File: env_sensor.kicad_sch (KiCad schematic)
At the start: 41 parts, among them J1 E Paper, J10 PWMOUT, J15 MH-Z19, J16 ADCs, J18 Conn_01x02_Pin, J3 Barrel_Jack, J4 LED_OUTPUT, J6 ADCs, J7 USB_C_Receptacle_USB2.0_16P, J8 v5_v3, J9 DEBUG, Q1 NMOS, Q2 NMOS, Q3 NMOS, SW1 EN, SW2 BOOT, U3 ESP32-S3-WROOM-1, U4 TXB0104PW, U6 TPS2065CDBV, U7 AP7361C-33E, Y1 Crystal

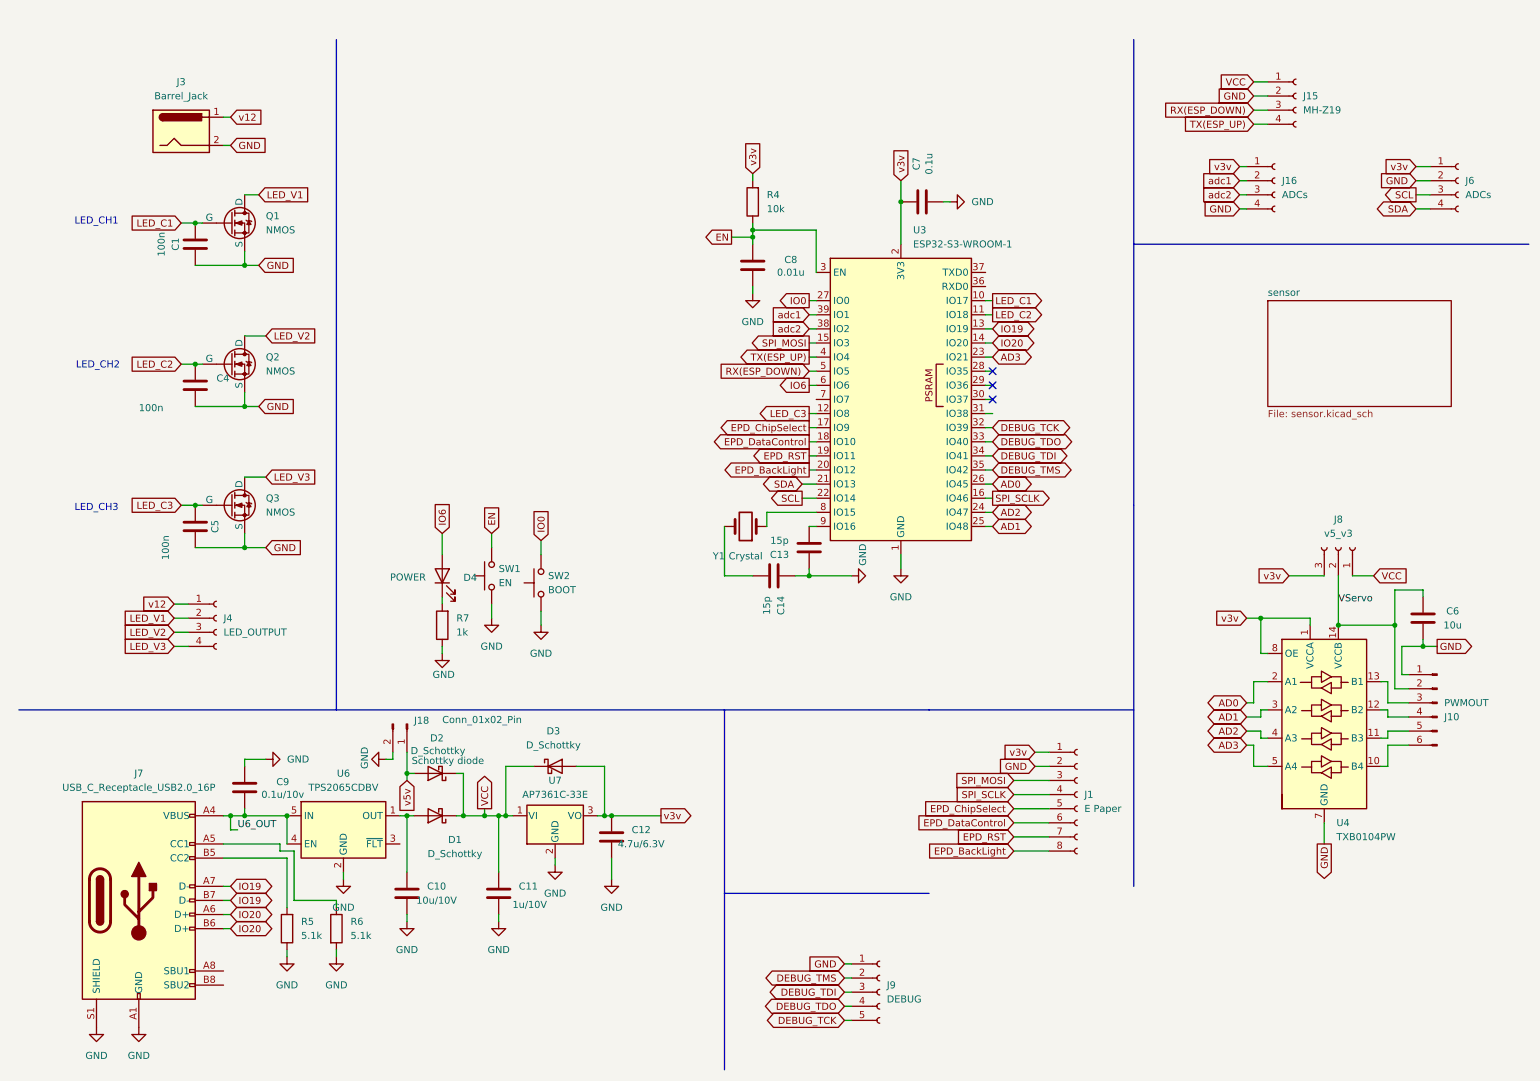
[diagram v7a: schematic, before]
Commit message: update
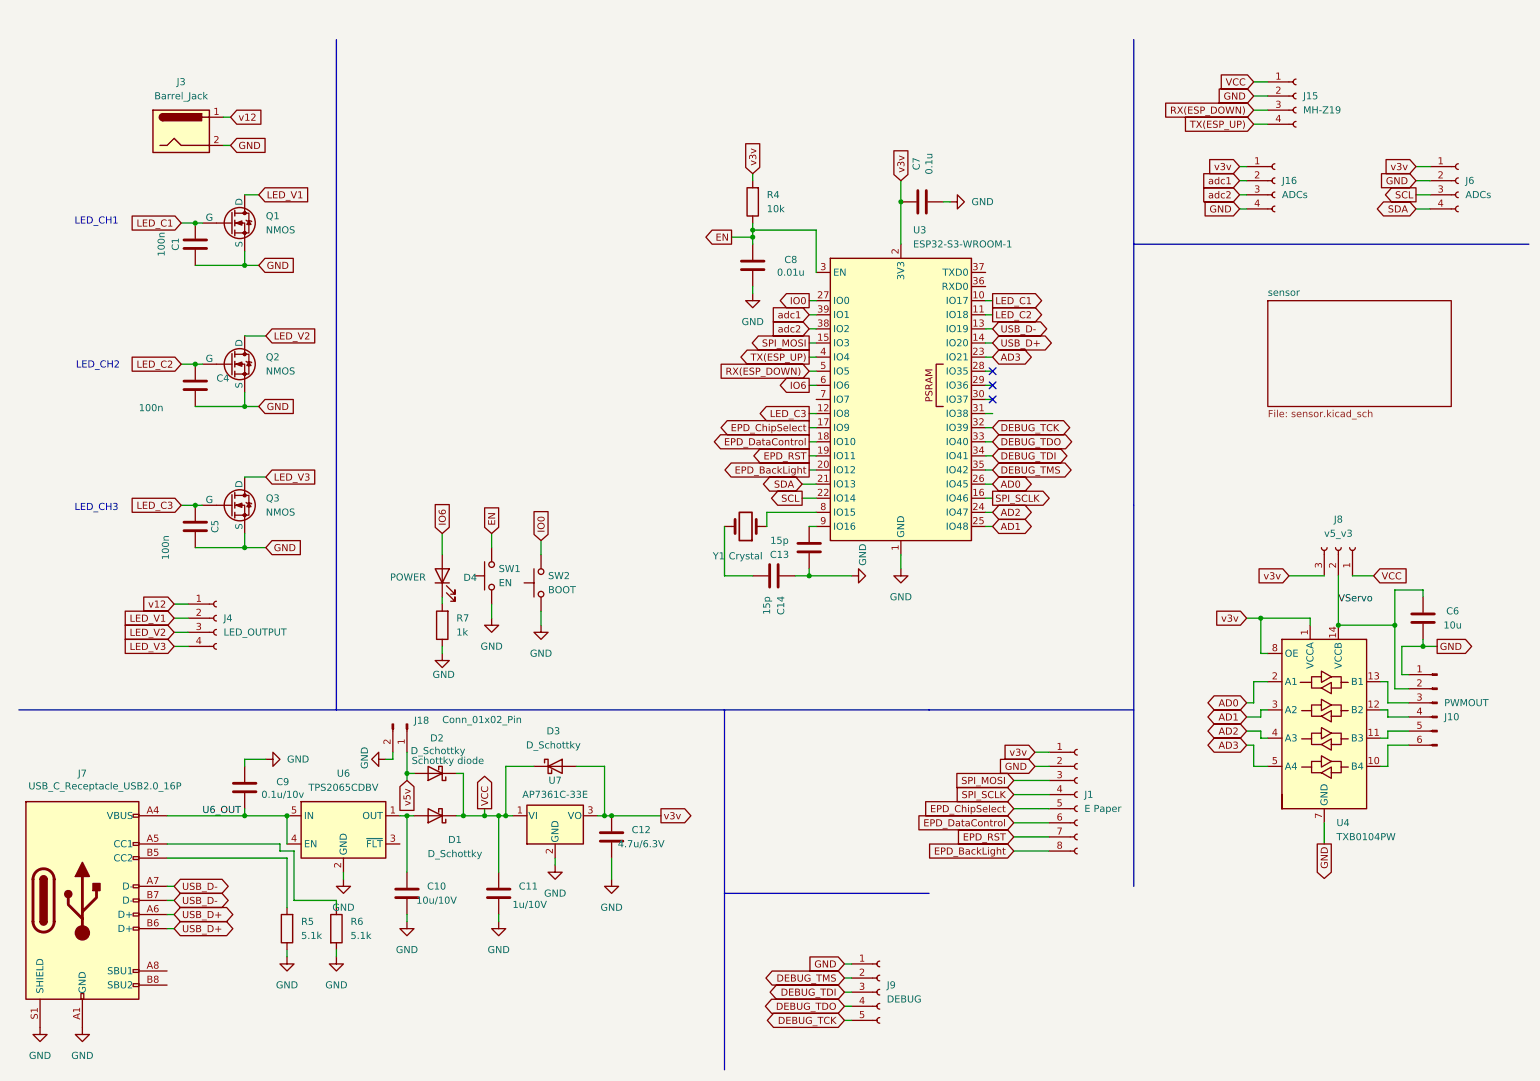
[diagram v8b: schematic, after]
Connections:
- net IO19 renamed USB_D-
- net IO20 renamed USB_D+
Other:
- moved on the sheet: J7
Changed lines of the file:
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@@
 	)
 	(junction
-		(at 50.8 152.4)
-		(diameter 0)
-		(color 0 0 0 0)
-	)
-	(junction
 		(at 171.45 41.91)
 		(diameter 0)
@@
 	(wire
 		(pts
-			(xy 50.8 165.1) (xy 49.53 165.1)
+			(xy 40.64 165.1) (xy 39.37 165.1)
 		)
 		(stroke
@@
 	(wire
 		(pts
-			(xy 53.34 152.4) (xy 50.8 152.4)
-		)
-		(stroke
-			(width 0)
-			(type default)
-		)
-	)
-	(wire
-		(pts
 			(xy 259.08 134.62) (xy 262.89 134.62)
 		)
@@
 	(wire
 		(pts
-			(xy 49.53 160.02) (xy 60.96 160.02)
+			(xy 39.37 160.02) (xy 60.96 160.02)
 		)
 		(stroke
@@
 	(wire
 		(pts
-			(xy 50.8 167.64) (xy 49.53 167.64)
+			(xy 40.64 167.64) (xy 39.37 167.64)
 		)
 		(stroke
@@
 	(wire
 		(pts
+			(xy 39.37 170.18) (xy 40.64 170.18)
+		)
+		(stroke
+			(width 0)
+			(type default)
+		)
+	)
+	(wire
+		(pts
 			(xy 236.22 123.19) (xy 236.22 116.84)
 		)
@@
 	(wire
 		(pts
-			(xy 50.8 172.72) (xy 49.53 172.72)
+			(xy 40.64 172.72) (xy 39.37 172.72)
 		)
 		(stroke
@@
 	(wire
 		(pts
-			(xy 50.8 154.94) (xy 50.8 152.4)
-		)
-		(stroke
-			(width 0)
-			(type default)
-		)
-	)
-	(wire
-		(pts
 			(xy 234.95 27.94) (xy 237.49 27.94)
 		)
@@
 	(wire
 		(pts
-			(xy 50.8 152.4) (xy 49.53 152.4)
+			(xy 39.37 152.4) (xy 53.34 152.4)
 		)
 		(stroke
@@
 	(wire
 		(pts
-			(xy 49.53 157.48) (xy 59.69 157.48)
+			(xy 39.37 157.48) (xy 59.69 157.48)
 		)
 		(stroke
@@
 	(wire
 		(pts
-			(xy 50.8 170.18) (xy 49.53 170.18)
-		)
-		(stroke
-			(width 0)
-			(type default)
-		)
-	)
-	(wire
-		(pts
 			(xy 53.34 76.2) (xy 53.34 78.74)
 		)
@@
 	(wire
 		(pts
-			(xy 52.07 154.94) (xy 50.8 154.94)
-		)
-		(stroke
-			(width 0)
-			(type default)
-		)
-	)
-	(wire
-		(pts
 			(xy 187.96 69.85) (xy 186.69 69.85)
 		)
@@
 	)
 	(label "U6_OUT"
-		(at 52.07 154.94 0)
+		(at 45.72 152.4 0)
 		(fields_autoplaced yes)
 		(effects
@@
 		)
 	)
-	(global_label "IO20"
+	(global_label "USB_D+"
 		(shape bidirectional)
 		(at 187.96 67.31 0)
@@
 		)
 	)
-	(global_label "IO19"
+	(global_label "USB_D-"
 		(shape bidirectional)
-		(at 50.8 167.64 0)
+		(at 40.64 167.64 0)
 		(fields_autoplaced yes)
 		(effects
@@
 		)
 		(property "Intersheetrefs" "${INTERSHEET_REFS}"
-			(at 59.2508 167.64 0)
+			(at 49.0908 167.64 0)
 			(effects
 				(font
@@
 		)
 	)
-	(global_label "IO19"
+	(global_label "USB_D-"
 		(shape bidirectional)
 		(at 187.96 64.77 0)
@@
 		)
 	)
-	(global_label "IO20"
+	(global_label "USB_D+"
 		(shape bidirectional)
-		(at 50.8 172.72 0)
+		(at 40.64 172.72 0)
 		(fields_autoplaced yes)
 		(effects
@@
 		)
 		(property "Intersheetrefs" "${INTERSHEET_REFS}"
-			(at 59.2508 172.72 0)
+			(at 49.0908 172.72 0)
 			(effects
 				(font
@@
 		)
 	)
-	(global_label "IO19"
+	(global_label "USB_D-"
 		(shape bidirectional)
-		(at 50.8 165.1 0)
+		(at 40.64 165.1 0)
 		(fields_autoplaced yes)
 		(effects
@@
 		)
 		(property "Intersheetrefs" "${INTERSHEET_REFS}"
-			(at 59.2508 165.1 0)
+			(at 49.0908 165.1 0)
 			(effects
 				(font
@@
 		)
 	)
-	(global_label "IO20"
+	(global_label "USB_D+"
 		(shape bidirectional)
-		(at 50.8 170.18 0)
+		(at 40.64 170.18 0)
 		(fields_autoplaced yes)
 		(effects
@@
 		)
 		(property "Intersheetrefs" "${INTERSHEET_REFS}"
-			(at 59.2508 170.18 0)
+			(at 49.0908 170.18 0)
 			(effects
 				(font
@@
 	(symbol
 		(lib_id "power:GND")
-		(at 26.67 190.5 0)
+		(at 16.51 190.5 0)
 		(unit 1)
 		(exclude_from_sim no)
@@
 		(fields_autoplaced yes)
 		(property "Reference" "#PWR02"
-			(at 26.67 196.85 0)
+			(at 16.51 196.85 0)
 			(effects
 				(font
@@
 		)
 		(property "Value" "GND"
-			(at 26.67 195.58 0)
+			(at 16.51 195.58 0)
 			(effects
 				(font
@@
 		)
 		(property "Footprint" ""
-			(at 26.67 190.5 0)
+			(at 16.51 190.5 0)
 			(effects
 				(font
@@
 		)
 		(property "Datasheet" ""
-			(at 26.67 190.5 0)
+			(at 16.51 190.5 0)
 			(effects
 				(font
@@
 		)
 		(property "Description" "Power symbol creates a global label with name \"GND\" , ground"
-			(at 26.67 190.5 0)
+			(at 16.51 190.5 0)
 			(effects
 				(font
@@
 	(symbol
 		(lib_id "power:GND")
-		(at 34.29 190.5 0)
+		(at 24.13 190.5 0)
 		(unit 1)
 		(exclude_from_sim no)
@@
 		(fields_autoplaced yes)
 		(property "Reference" "#PWR03"
-			(at 34.29 196.85 0)
+			(at 24.13 196.85 0)
 			(effects
 				(font
@@
 		)
 		(property "Value" "GND"
-			(at 34.29 195.58 0)
+			(at 24.13 195.58 0)
 			(effects
 				(font
@@
 		)
 		(property "Footprint" ""
-			(at 34.29 190.5 0)
+			(at 24.13 190.5 0)
 			(effects
 				(font
@@
 		)
 		(property "Datasheet" ""
-			(at 34.29 190.5 0)
+			(at 24.13 190.5 0)
 			(effects
 				(font
@@
 		)
 		(property "Description" "Power symbol creates a global label with name \"GND\" , ground"
-			(at 34.29 190.5 0)
+			(at 24.13 190.5 0)
 			(effects
 				(font
@@
 	(symbol
 		(lib_id "Connector:USB_C_Receptacle_USB2.0_16P")
-		(at 34.29 167.64 0)
+		(at 24.13 167.64 0)
 		(unit 1)
 		(exclude_from_sim no)
@@
 		(on_board yes)
 		(dnp no)
-		(fields_autoplaced yes)
 		(property "Reference" "J7"
-			(at 34.29 144.78 0)
+			(at 24.13 144.78 0)
 			(effects
 				(font
@@
 		)
 		(property "Value" "USB_C_Receptacle_USB2.0_16P"
-			(at 34.29 147.32 0)
+			(at 28.194 147.066 0)
 			(effects
 				(font
@@
 		)
 		(property "Footprint" "Connector_USB:USB_C_Receptacle_GCT_USB4085"
-			(at 38.1 167.64 0)
+			(at 27.94 167.64 0)
 			(effects
 				(font
@@
 		)
 		(property "Datasheet" "https://www.usb.org/sites/default/files/documents/usb_type-c.zip"
-			(at 38.1 167.64 0)
+			(at 27.94 167.64 0)
 			(effects
 				(font
@@
 		)
 		(property "Description" "USB 2.0-only 16P Type-C Receptacle connector"
-			(at 34.29 167.64 0)
+			(at 24.13 167.64 0)
 			(effects
 				(font
@@
 		)
 		(property "LCSC" "C7095263"
-			(at 34.29 167.64 0)
+			(at 24.13 167.64 0)
 			(effects
 				(font
